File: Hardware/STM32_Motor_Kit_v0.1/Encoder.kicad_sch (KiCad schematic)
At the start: 21 parts, among them J5 Conn_01x06_Male

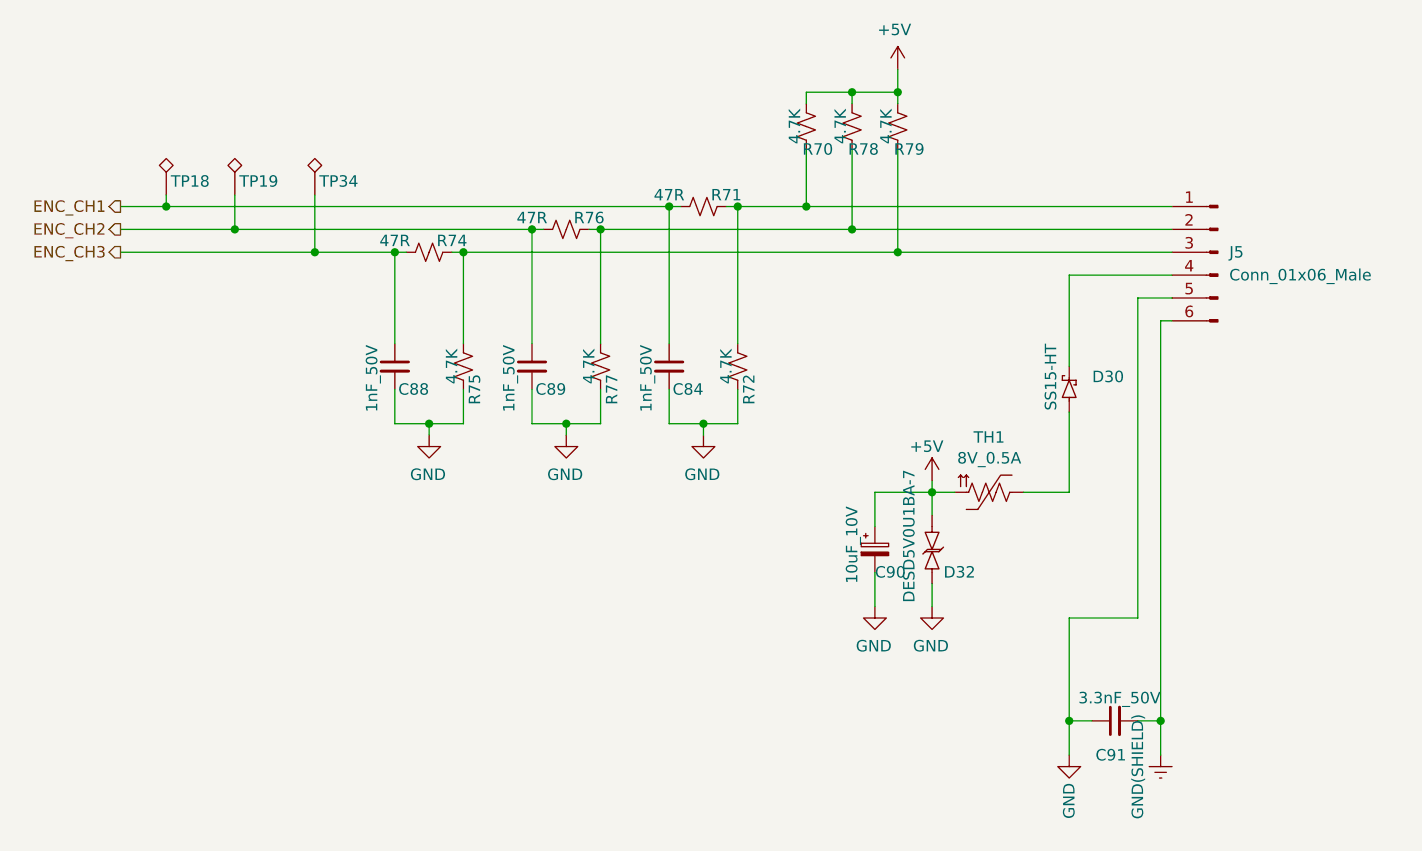
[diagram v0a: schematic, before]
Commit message: 12.01.2025
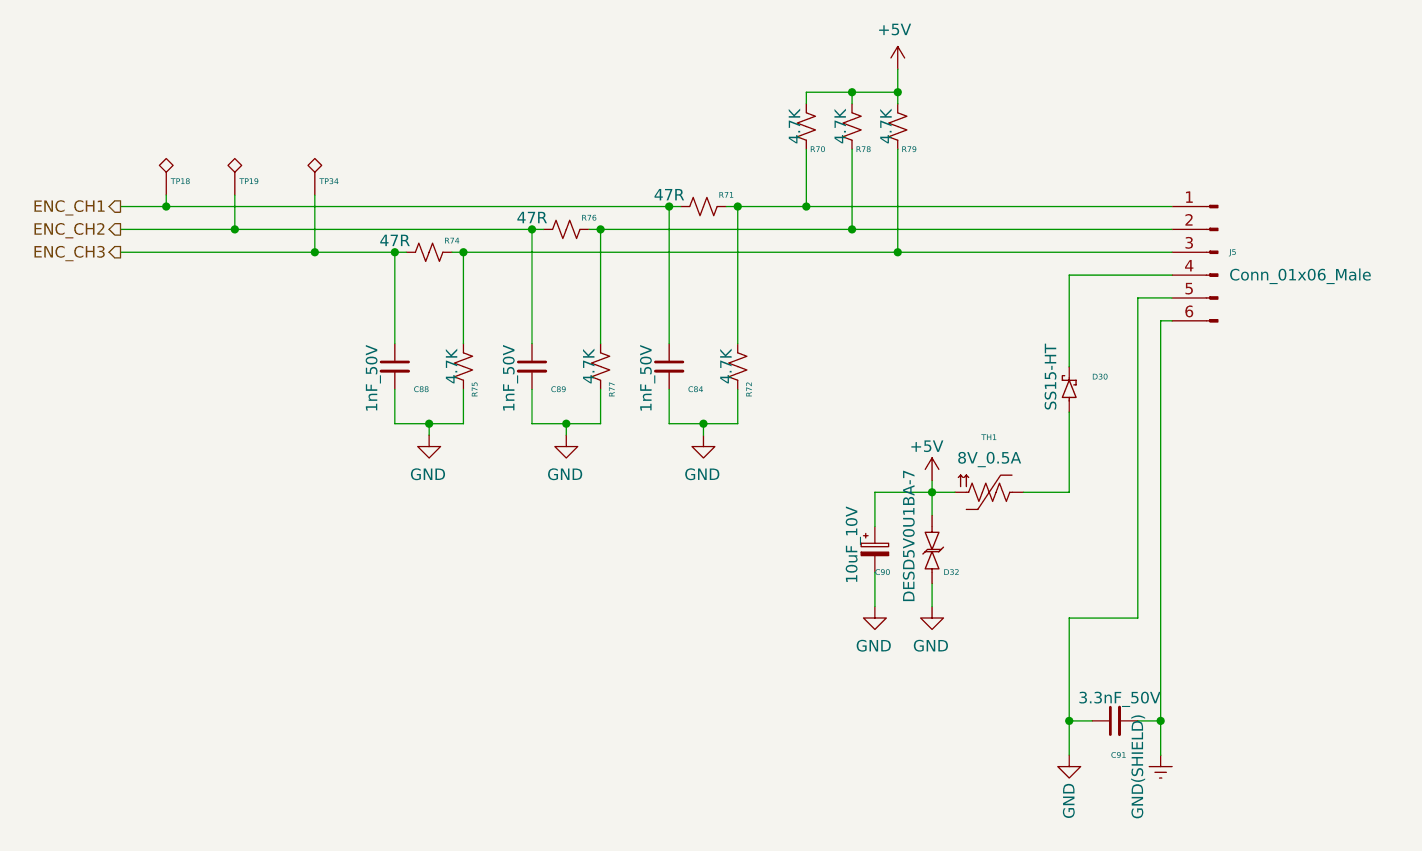
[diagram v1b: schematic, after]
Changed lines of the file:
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@@
 			(effects
 				(font
-					(size 1.27 1.27)
+					(face "Arial")
+					(size 0.635 0.635)
 				)
 				(justify left)
@@
 			(effects
 				(font
-					(size 1.27 1.27)
+					(face "Arial")
+					(size 0.635 0.635)
 				)
 				(hide yes)
@@
 			(effects
 				(font
-					(size 1.27 1.27)
+					(face "Arial")
+					(size 0.635 0.635)
 				)
 				(justify left)
@@
 			(effects
 				(font
-					(size 1.27 1.27)
+					(face "Arial")
+					(size 0.635 0.635)
 				)
 				(hide yes)
@@
 			(effects
 				(font
-					(size 1.27 1.27)
+					(face "Arial")
+					(size 0.635 0.635)
 				)
 				(justify left)
@@
 			(effects
 				(font
-					(size 1.27 1.27)
+					(face "Arial")
+					(size 0.635 0.635)
 				)
 				(hide yes)
@@
 			(effects
 				(font
-					(size 1.27 1.27)
+					(face "Arial")
+					(size 0.635 0.635)
 				)
 			)
@@
 			(effects
 				(font
-					(size 1.27 1.27)
+					(face "Arial")
+					(size 0.635 0.635)
 				)
 				(justify left)
@@
 			(effects
 				(font
-					(size 1.27 1.27)
+					(face "Arial")
+					(size 0.635 0.635)
 				)
 				(justify left)
@@
 			(effects
 				(font
-					(size 1.27 1.27)
+					(face "Arial")
+					(size 0.635 0.635)
 				)
 				(hide yes)
@@
 			(effects
 				(font
-					(size 1.27 1.27)
+					(face "Arial")
+					(size 0.635 0.635)
 				)
 				(justify left)
@@
 			(effects
 				(font
-					(size 1.27 1.27)
+					(face "Arial")
+					(size 0.635 0.635)
 				)
 			)
@@
 			(effects
 				(font
-					(size 1.27 1.27)
+					(face "Arial")
+					(size 0.635 0.635)
 				)
 				(justify left)
@@
 			(effects
 				(font
-					(size 1.27 1.27)
+					(face "Arial")
+					(size 0.635 0.635)
 				)
 				(hide yes)
@@
 			(effects
 				(font
-					(size 1.27 1.27)
+					(face "Arial")
+					(size 0.635 0.635)
 				)
 				(hide yes)
@@
 			(effects
 				(font
-					(size 1.27 1.27)
+					(face "Arial")
+					(size 0.635 0.635)
 				)
 				(hide yes)
@@
 			(effects
 				(font
-					(size 1.27 1.27)
+					(face "Arial")
+					(size 0.635 0.635)
 				)
 			)
@@
 			(effects
 				(font
-					(size 1.27 1.27)
+					(face "Arial")
+					(size 0.635 0.635)
 				)
 				(justify left)
@@
 			(effects
 				(font
-					(size 1.27 1.27)
+					(face "Arial")
+					(size 0.635 0.635)
 				)
 			)
@@
 			(effects
 				(font
-					(size 1.27 1.27)
+					(face "Arial")
+					(size 0.635 0.635)
 				)
 				(hide yes)
@@
 			(effects
 				(font
-					(size 1.27 1.27)
+					(face "Arial")
+					(size 0.635 0.635)
 				)
 			)
@@
 			(effects
 				(font
-					(size 1.27 1.27)
+					(face "Arial")
+					(size 0.635 0.635)
 				)
 			)
@@
 			(effects
 				(font
-					(size 1.27 1.27)
+					(face "Arial")
+					(size 0.635 0.635)
 				)
 				(justify right)
@@
 			(effects
 				(font
-					(size 1.27 1.27)
+					(face "Arial")
+					(size 0.635 0.635)
 				)
 			)
@@
 			(effects
 				(font
-					(size 1.27 1.27)
+					(face "Arial")
+					(size 0.635 0.635)
 				)
 			)
@@
 			(effects
 				(font
-					(size 1.27 1.27)
+					(face "Arial")
+					(size 0.635 0.635)
 				)
 			)
@@
 			(effects
 				(font
-					(size 1.27 1.27)
+					(face "Arial")
+					(size 0.635 0.635)
 				)
 				(justify left)
@@
 			(effects
 				(font
-					(size 1.27 1.27)
+					(face "Arial")
+					(size 0.635 0.635)
 				)
 				(justify left)
@@
 			(effects
 				(font
-					(size 1.27 1.27)
+					(face "Arial")
+					(size 0.635 0.635)
 				)
 				(hide yes)
@@
 			(effects
 				(font
-					(size 1.27 1.27)
-				)
-			)
+					(face "Arial")
+					(size 0.635 0.635)
+				)
+			)
